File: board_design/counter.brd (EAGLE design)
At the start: 54.3 x 94 mm, 24 parts, among them IC1 7805T

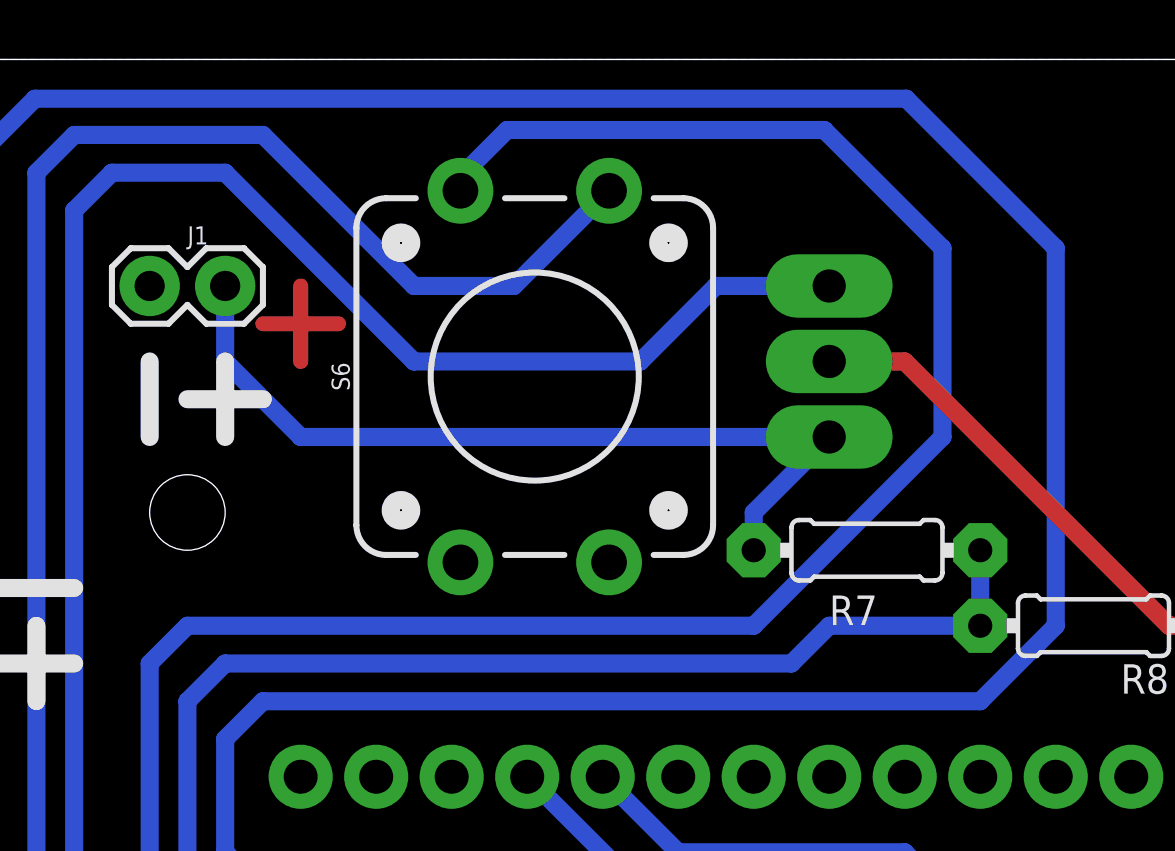
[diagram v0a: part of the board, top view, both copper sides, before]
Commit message: couple changes to board
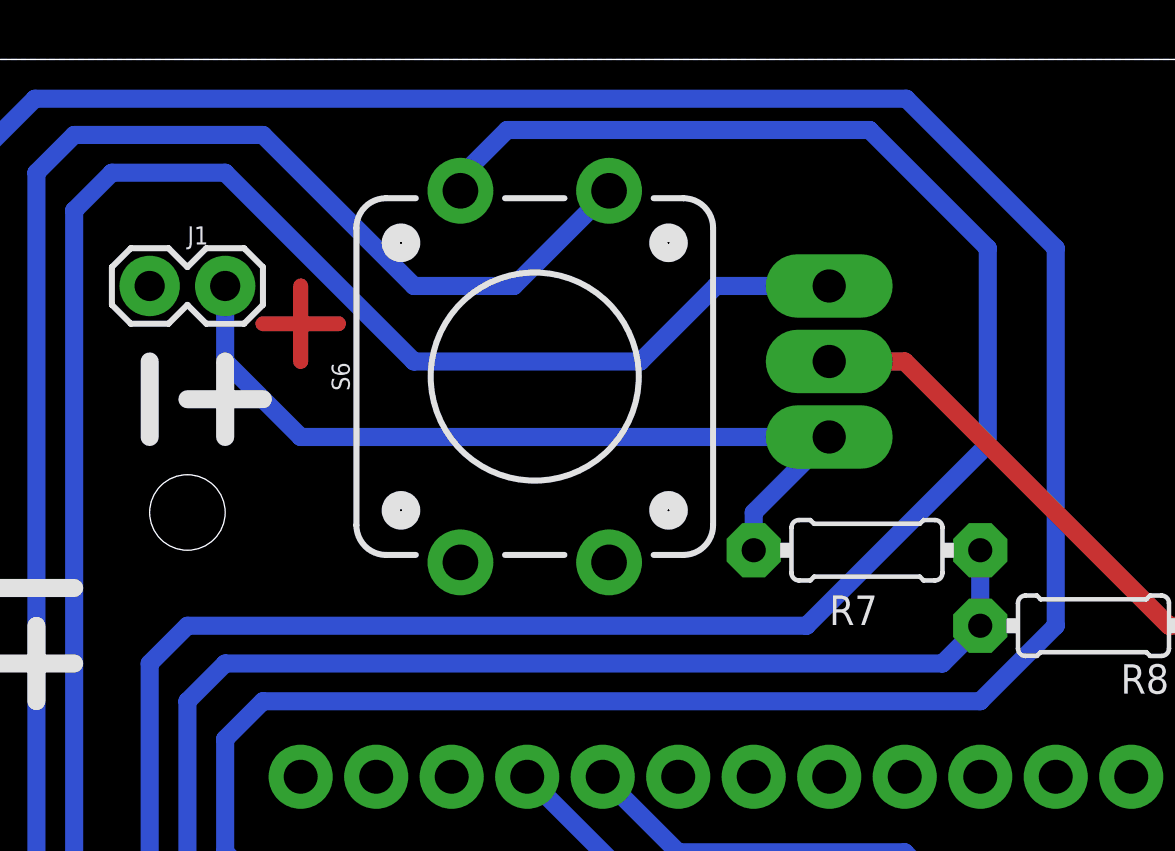
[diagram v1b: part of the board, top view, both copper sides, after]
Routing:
- net CLR: track 92.2 -> 95.4 mm
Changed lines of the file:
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@@
 <wire x1="23.154" y1="89.562" x2="23.154" y2="90.037225" width="0.6096" layer="16"/>
 <wire x1="23.154" y1="90.037225" x2="24.723475" y2="91.6067" width="0.6096" layer="16"/>
-<wire x1="24.723475" y1="91.6067" x2="35.3933" y2="91.6067" width="0.6096" layer="16"/>
-<wire x1="35.3933" y1="91.6067" x2="39.37" y2="87.63" width="0.6096" layer="16"/>
-<wire x1="39.37" y1="87.63" x2="39.37" y2="81.28" width="0.6096" layer="16"/>
-<wire x1="39.37" y1="81.28" x2="33.02" y2="74.93" width="0.6096" layer="16"/>
-<wire x1="33.02" y1="74.93" x2="13.97" y2="74.93" width="0.6096" layer="16"/>
+<wire x1="24.723475" y1="91.6067" x2="36.9173" y2="91.6067" width="0.6096" layer="16"/>
+<wire x1="36.9173" y1="91.6067" x2="40.894" y2="87.63" width="0.6096" layer="16"/>
+<wire x1="40.894" y1="87.63" x2="40.894" y2="81.026" width="0.6096" layer="16"/>
+<wire x1="40.894" y1="81.026" x2="34.798" y2="74.93" width="0.6096" layer="16"/>
+<wire x1="34.798" y1="74.93" x2="13.97" y2="74.93" width="0.6096" layer="16"/>
 <wire x1="13.97" y1="74.93" x2="12.7" y2="73.66" width="0.6096" layer="16"/>
 <wire x1="12.7" y1="57.15" x2="22.86" y2="46.99" width="0.6096" layer="16"/>
@@
 <contactref element="R8" pad="2"/>
 <wire x1="40.64" y1="77.47" x2="40.64" y2="74.93" width="0.6096" layer="16"/>
-<wire x1="40.64" y1="74.93" x2="35.56" y2="74.93" width="0.6096" layer="16"/>
+<wire x1="40.64" y1="74.93" x2="39.37" y2="73.66" width="0.6096" layer="16"/>
 <contactref element="U$1" pad="33"/>
-<wire x1="35.56" y1="74.93" x2="34.29" y2="73.66" width="0.6096" layer="16"/>
-<wire x1="34.29" y1="73.66" x2="15.24" y2="73.66" width="0.6096" layer="16"/>
+<wire x1="39.37" y1="73.66" x2="15.24" y2="73.66" width="0.6096" layer="16"/>
 <wire x1="15.24" y1="73.66" x2="13.97" y2="72.39" width="0.6096" layer="16"/>
 <wire x1="13.97" y1="72.39" x2="13.97" y2="66.04" width="0.6096" layer="16"/>
